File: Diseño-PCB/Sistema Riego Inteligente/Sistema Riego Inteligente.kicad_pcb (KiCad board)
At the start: 2 copper layers, 7 parts, among them J1 electroválvula, U1 DEVKIT_V1_ESP32-WROOM-32, U2 DHT11

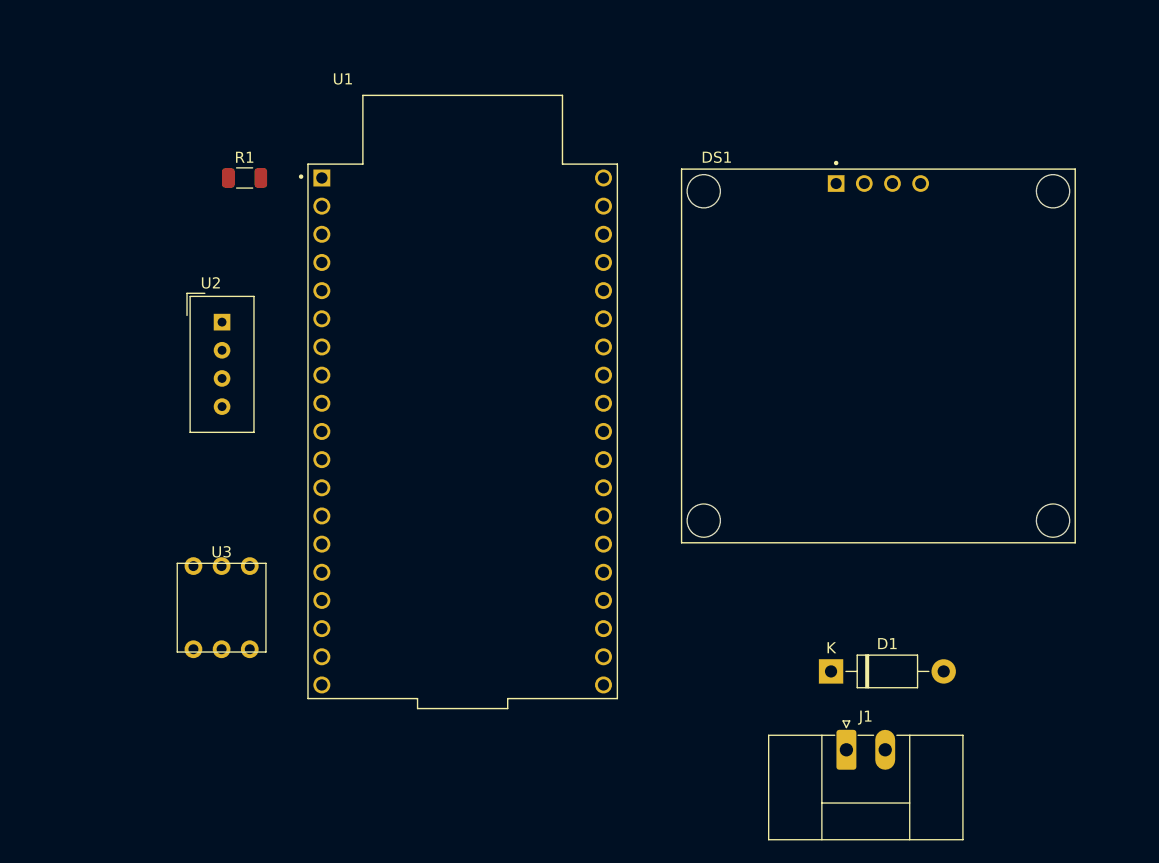
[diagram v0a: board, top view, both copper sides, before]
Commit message: Completo ruteo y diseño de PCB
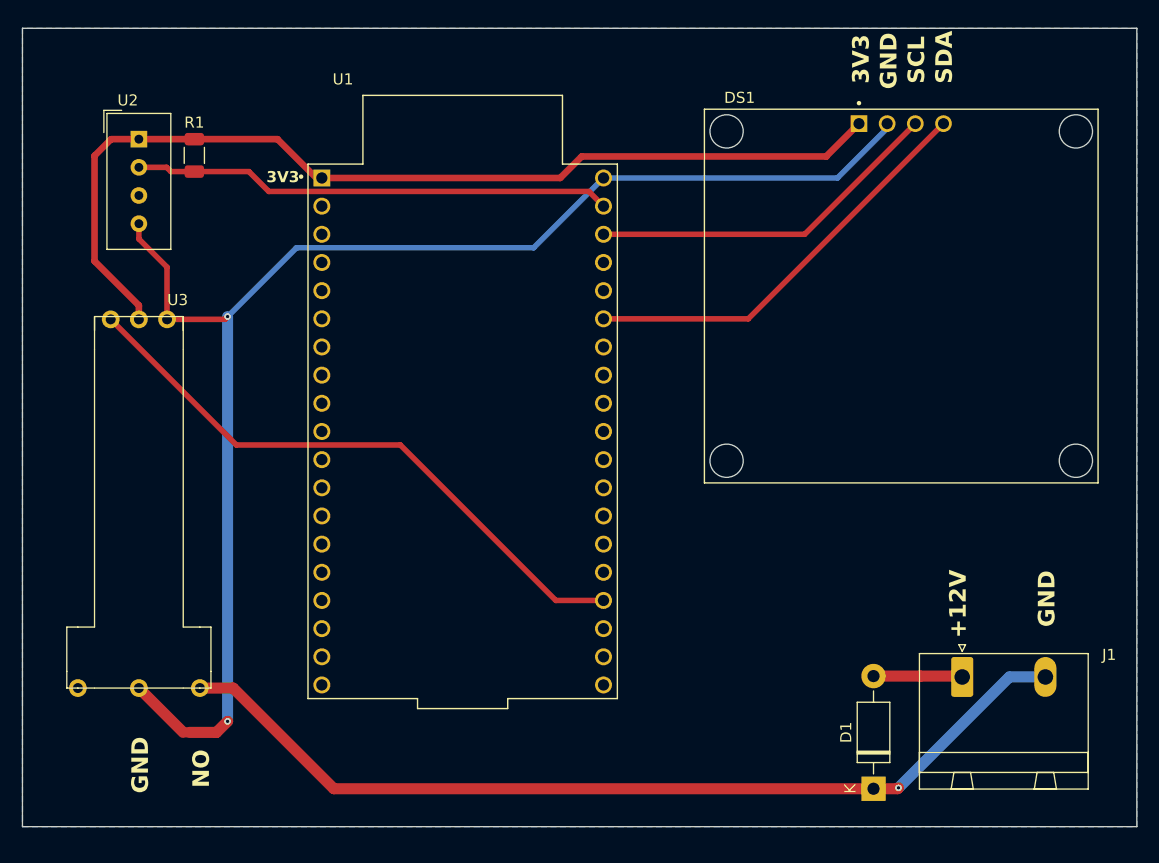
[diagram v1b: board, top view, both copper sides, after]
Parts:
- J1: footprint Connector_Phoenix_MC:PhoenixContact_MC_1,5_2-GF-3.5_1x02_P3.50mm_Horizontal_ThreadedFlange -> Connector_Phoenix_GMSTB:PhoenixContact_GMSTBA_2,5_2-G_1x02_P7.50mm_Horizontal
- moved U2 18.1 mm to (82.0, 66.5)
- moved J1 12.3 mm to (156.2, 115.0)
- moved U3 11.9 mm to (82.0, 99.5)
- moved D1 11.3 mm to (148.2, 125.1), turned to 90 degrees
- moved DS1 5.78 mm to (150.8, 80.7)
- moved R1 4.97 mm to (87.0, 68.0), turned to 90 degrees
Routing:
- net GND: track 0.00 -> 128.8 mm, vias 0 -> 2
- net /3v3: track 0.00 -> 89.5 mm
- net Net-(D1-K): track 0.00 -> 84.2 mm, vias 0 -> 1
- net /RELE_CTRL: track 0.00 -> 54.9 mm
- net /DATA: track 0.00 -> 43.3 mm
- net /SDA: track 0.00 -> 38.0 mm
- net /SCL: track 0.00 -> 32.3 mm
- net +12V: track 0.00 -> 8.03 mm
- added copper zone on B.Cu, net GND
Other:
- board outline added: 100.5 x 72 mm
- board text added: "+12V"
- board text added: "3V3"
- board text added: "GND"
- board text added: "NO"
- board text added: "SCL"
- board text added: "SDA"
